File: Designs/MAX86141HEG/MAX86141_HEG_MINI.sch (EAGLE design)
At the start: 19 parts, among them U1 MAX86141ENP+T, U3 TXBN0304RUTR, U4 LP5907MFX-3.3/NOPB

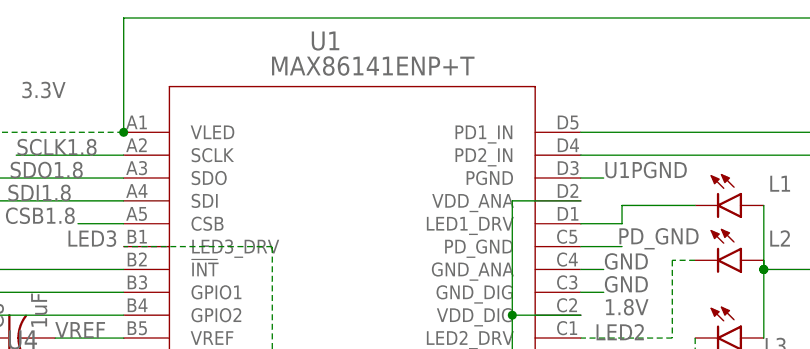
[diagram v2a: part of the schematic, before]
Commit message: reverted breakout board (trace spacing too narrow)
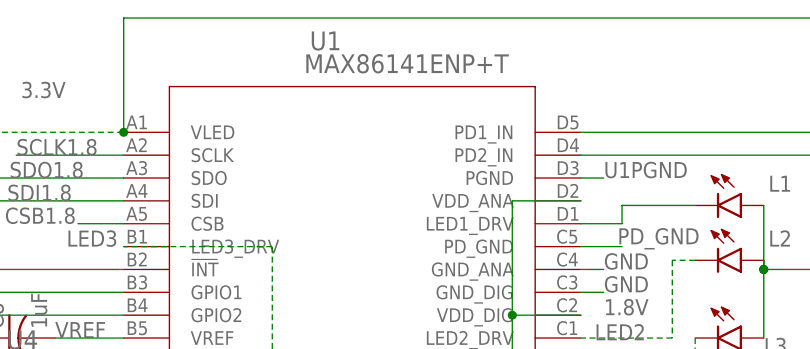
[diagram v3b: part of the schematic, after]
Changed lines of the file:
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@@
 <?xml version="1.0" encoding="utf-8"?>
 <!DOCTYPE eagle SYSTEM "eagle.dtd">
-<eagle version="9.6.2">
+<eagle version="9.5.1">
 <drawing>
 <settings>
@@
 <grid distance="10" unitdist="mil" unit="mil" style="lines" multiple="1" display="no" altdistance="0.01" altunitdist="inch" altunit="inch"/>
 <layers>
-<layer number="1" name="Top" color="4" fill="1" visible="yes" active="no"/>
-<layer number="2" name="Route2" color="16" fill="1" visible="yes" active="no"/>
-<layer number="3" name="Route3" color="17" fill="1" visible="yes" active="no"/>
-<layer number="4" name="Route4" color="18" fill="1" visible="yes" active="no"/>
-<layer number="5" name="Route5" color="19" fill="1" visible="yes" active="no"/>
-<layer number="6" name="Route6" color="25" fill="1" visible="yes" active="no"/>
-<layer number="7" name="Route7" color="26" fill="1" visible="yes" active="no"/>
-<layer number="8" name="Route8" color="27" fill="1" visible="yes" active="no"/>
-<layer number="9" name="Route9" color="28" fill="1" visible="yes" active="no"/>
-<layer number="10" name="Route10" color="29" fill="1" visible="yes" active="no"/>
-<layer number="11" name="Route11" color="30" fill="1" visible="yes" active="no"/>
-<layer number="12" name="Route12" color="20" fill="1" visible="yes" active="no"/>
-<layer number="13" name="Route13" color="21" fill="1" visible="yes" active="no"/>
-<layer number="14" name="Route14" color="22" fill="1" visible="yes" active="no"/>
-<layer number="15" name="Route15" color="23" fill="1" visible="yes" active="no"/>
-<layer number="16" name="Bottom" color="1" fill="1" visible="yes" active="no"/>
-<layer number="17" name="Pads" color="2" fill="1" visible="yes" active="no"/>
-<layer number="18" name="Vias" color="2" fill="1" visible="yes" active="no"/>
-<layer number="19" name="Unrouted" color="6" fill="1" visible="yes" active="no"/>
-<layer number="20" name="Dimension" color="24" fill="1" visible="yes" active="no"/>
-<layer number="21" name="tPlace" color="7" fill="1" visible="yes" active="no"/>
-<layer number="22" name="bPlace" color="7" fill="1" visible="yes" active="no"/>
-<layer number="23" name="tOrigins" color="15" fill="1" visible="yes" active="no"/>
-<layer number="24" name="bOrigins" color="15" fill="1" visible="yes" active="no"/>
-<layer number="25" name="tNames" color="7" fill="1" visible="yes" active="no"/>
-<layer number="26" name="bNames" color="7" fill="1" visible="yes" active="no"/>
-<layer number="27" name="tValues" color="7" fill="1" visible="yes" active="no"/>
-<layer number="28" name="bValues" color="7" fill="1" visible="yes" active="no"/>
+<layer number="1" name="Top" color="4" fill="1" visible="no" active="no"/>
+<layer number="2" name="Route2" color="1" fill="3" visible="no" active="no"/>
+<layer number="3" name="Route3" color="4" fill="3" visible="no" active="no"/>
+<layer number="4" name="Route4" color="1" fill="4" visible="no" active="no"/>
+<layer number="5" name="Route5" color="4" fill="4" visible="no" active="no"/>
+<layer number="6" name="Route6" color="1" fill="8" visible="no" active="no"/>
+<layer number="7" name="Route7" color="4" fill="8" visible="no" active="no"/>
+<layer number="8" name="Route8" color="1" fill="2" visible="no" active="no"/>
+<layer number="9" name="Route9" color="4" fill="2" visible="no" active="no"/>
+<layer number="10" name="Route10" color="1" fill="7" visible="no" active="no"/>
+<layer number="11" name="Route11" color="4" fill="7" visible="no" active="no"/>
+<layer number="12" name="Route12" color="1" fill="5" visible="no" active="no"/>
+<layer number="13" name="Route13" color="4" fill="5" visible="no" active="no"/>
+<layer number="14" name="Route14" color="1" fill="6" visible="no" active="no"/>
+<layer number="15" name="Route15" color="4" fill="6" visible="no" active="no"/>
+<layer number="16" name="Bottom" color="1" fill="1" visible="no" active="no"/>
+<layer number="17" name="Pads" color="2" fill="1" visible="no" active="no"/>
+<layer number="18" name="Vias" color="2" fill="1" visible="no" active="no"/>
+<layer number="19" name="Unrouted" color="6" fill="1" visible="no" active="no"/>
+<layer number="20" name="Dimension" color="24" fill="1" visible="no" active="no"/>
+<layer number="21" name="tPlace" color="7" fill="1" visible="no" active="no"/>
+<layer number="22" name="bPlace" color="7" fill="1" visible="no" active="no"/>
+<layer number="23" name="tOrigins" color="15" fill="1" visible="no" active="no"/>
+<layer number="24" name="bOrigins" color="15" fill="1" visible="no" active="no"/>
+<layer number="25" name="tNames" color="7" fill="1" visible="no" active="no"/>
+<layer number="26" name="bNames" color="7" fill="1" visible="no" active="no"/>
+<layer number="27" name="tValues" color="7" fill="1" visible="no" active="no"/>
+<layer number="28" name="bValues" color="7" fill="1" visible="no" active="no"/>
 <layer number="29" name="tStop" color="7" fill="3" visible="no" active="no"/>
 <layer number="30" name="bStop" color="7" fill="6" visible="no" active="no"/>
@@
 <layer number="35" name="tGlue" color="7" fill="4" visible="no" active="no"/>
 <layer number="36" name="bGlue" color="7" fill="5" visible="no" active="no"/>
-<layer number="37" name="tTest" color="7" fill="1" visible="yes" active="no"/>
-<layer number="38" name="bTest" color="7" fill="1" visible="yes" active="no"/>
+<layer number="37" name="tTest" color="7" fill="1" visible="no" active="no"/>
+<layer number="38" name="bTest" color="7" fill="1" visible="no" active="no"/>
 <layer number="39" name="tKeepout" color="4" fill="11" visible="no" active="no"/>
 <layer number="40" name="bKeepout" color="1" fill="11" visible="no" active="no"/>
@@
 <layer number="44" name="Drills" color="7" fill="1" visible="no" active="no"/>
 <layer number="45" name="Holes" color="7" fill="1" visible="no" active="no"/>
-<layer number="46" name="Milling" color="3" fill="1" visible="yes" active="no"/>
-<layer number="47" name="Measures" color="7" fill="1" visible="yes" active="no"/>
-<layer number="48" name="Document" color="7" fill="1" visible="yes" active="no"/>
-<layer number="49" name="Reference" color="7" fill="1" visible="yes" active="no"/>
-<layer number="50" name="dxf" color="7" fill="1" visible="yes" active="no"/>
-<layer number="51" name="tDocu" color="7" fill="1" visible="yes" active="no"/>
-<layer number="52" name="bDocu" color="7" fill="1" visible="yes" active="no"/>
-<layer number="53" name="tGND_GNDA" color="7" fill="9" visible="yes" active="no"/>
-<layer number="54" name="bGND_GNDA" color="1" fill="9" visible="yes" active="no"/>
-<layer number="56" name="wert" color="7" fill="1" visible="yes" active="no"/>
-<layer number="57" name="tCAD" color="7" fill="1" visible="yes" active="no"/>
-<layer number="59" name="tCarbon" color="7" fill="1" visible="yes" active="no"/>
-<layer number="60" name="bCarbon" color="7" fill="1" visible="yes" active="no"/>
+<layer number="46" name="Milling" color="3" fill="1" visible="no" active="no"/>
+<layer number="47" name="Measures" color="7" fill="1" visible="no" active="no"/>
+<layer number="48" name="Document" color="7" fill="1" visible="no" active="no"/>
+<layer number="49" name="Reference" color="7" fill="1" visible="no" active="no"/>
+<layer number="50" name="dxf" color="7" fill="1" visible="no" active="no"/>
+<layer number="51" name="tDocu" color="7" fill="1" visible="no" active="no"/>
+<layer number="52" name="bDocu" color="7" fill="1" visible="no" active="no"/>
+<layer number="53" name="tGND_GNDA" color="7" fill="9" visible="no" active="no"/>
+<layer number="54" name="bGND_GNDA" color="1" fill="9" visible="no" active="no"/>
+<layer number="56" name="wert" color="7" fill="1" visible="no" active="no"/>
+<layer number="57" name="tCAD" color="7" fill="1" visible="no" active="no"/>
+<layer number="59" name="tCarbon" color="7" fill="1" visible="no" active="no"/>
+<layer number="60" name="bCarbon" color="7" fill="1" visible="no" active="no"/>
 <layer number="88" name="SimResults" color="9" fill="1" visible="yes" active="yes"/>
 <layer number="89" name="SimProbes" color="9" fill="1" visible="yes" active="yes"/>
@@
 <instance part="U1" gate="A" x="43.18" y="96.52" smashed="yes">
 <attribute name="NAME" x="66.3956" y="105.6386" size="2.0828" layer="95" ratio="6" rot="SR0"/>
-<attribute name="VALUE" x="61.9506" y="102.8446" size="2.0828" layer="96" ratio="6" rot="SR0"/>
+<attribute name="VALUE" x="65.7606" y="103.0986" size="2.0828" layer="96" ratio="6" rot="SR0"/>
 </instance>
 <instance part="L2" gate="G$1" x="114.3" y="82.296" smashed="yes" rot="R270">
